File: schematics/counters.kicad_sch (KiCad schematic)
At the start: 28 parts, among them U10 74HC390, U11 74HC390, U12 74HC390, U13 ATF22V10C, U4 74HC08, U5 74HC08, U6 74HC4046, U7 74HC86, U8 74HC390, U9 74HC390

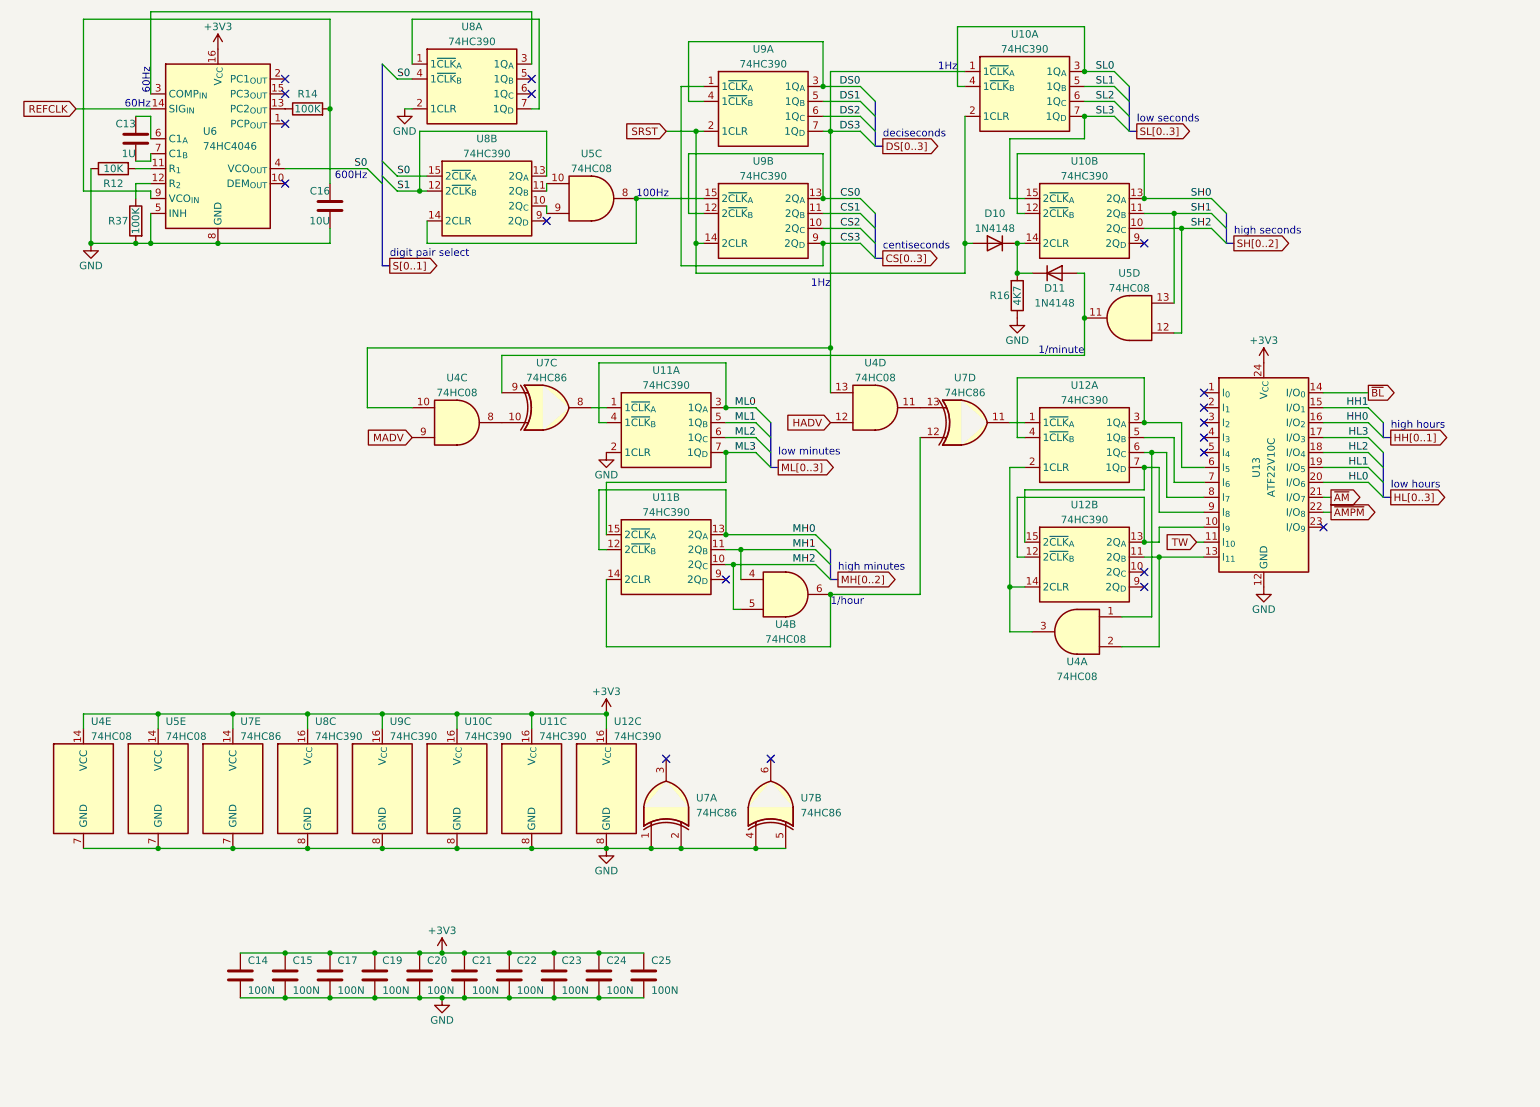
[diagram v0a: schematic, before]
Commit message: started a second version
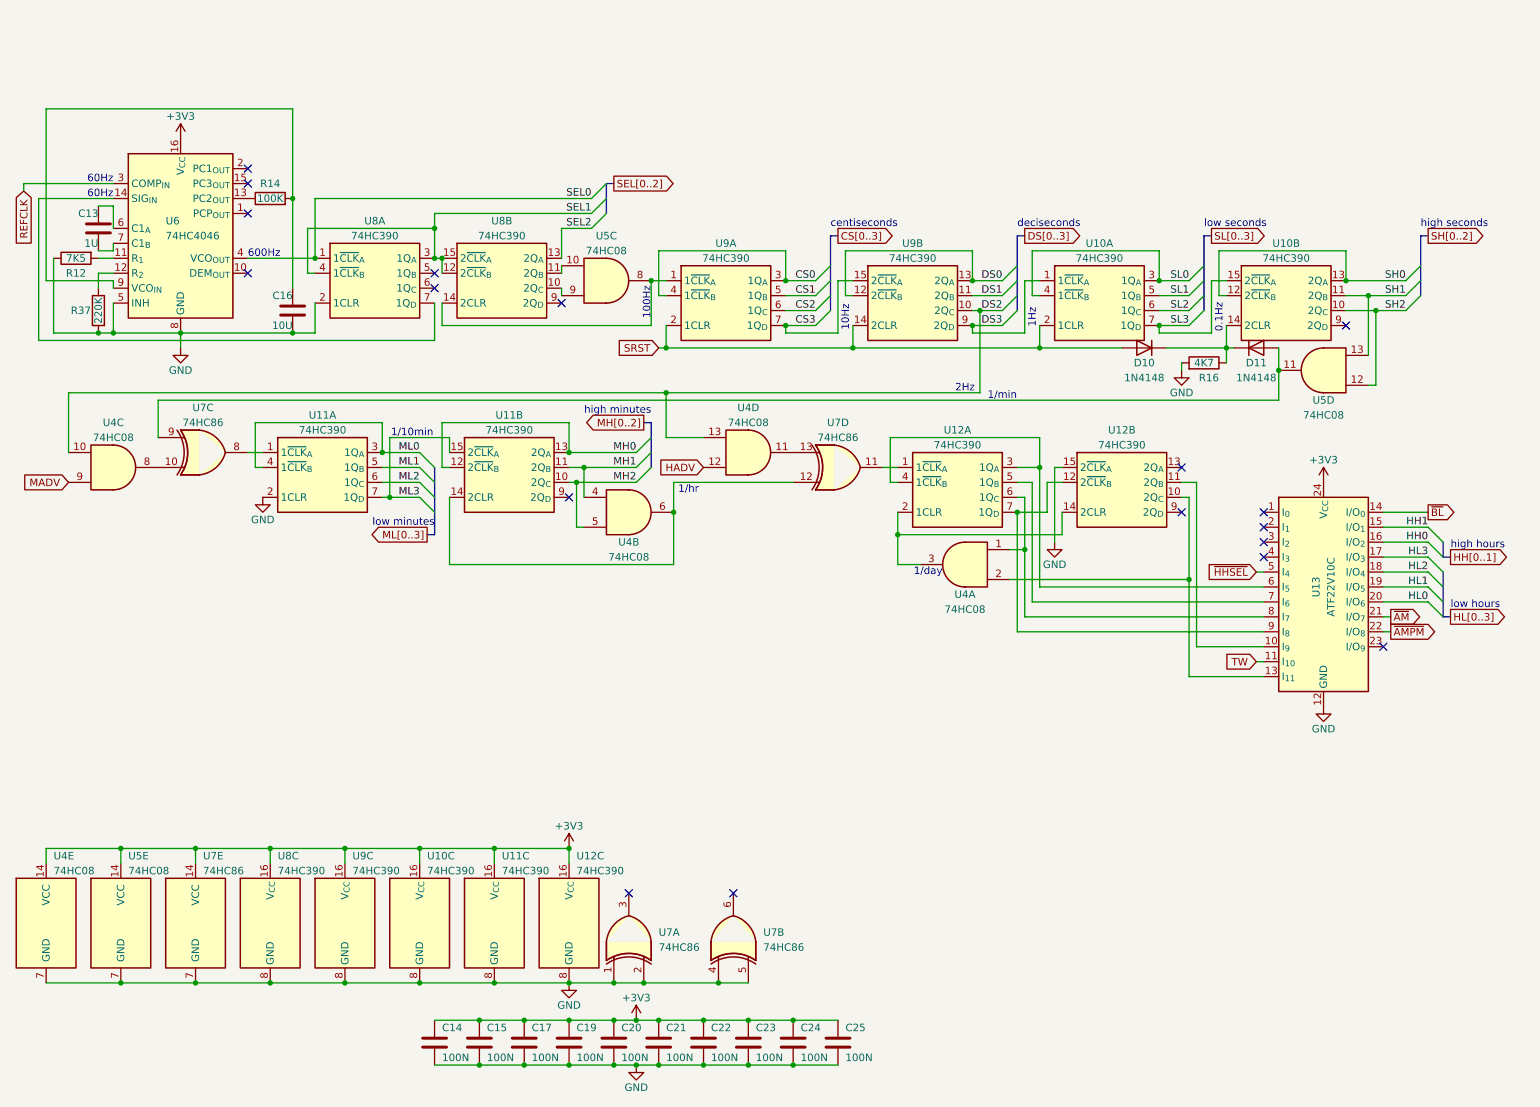
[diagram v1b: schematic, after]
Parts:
- R12: value 10K -> 7K5
- R37: value 100K -> 220K
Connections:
- net CS0: now also U9.3 (1Q_{A}), U9.4 (1~{CLK}_{B}); no longer U9.12 (2~{CLK}_{B}), U9.13 (2Q_{A})
- net CS1: now also U9.5 (1Q_{B}); no longer U9.11 (2Q_{B})
- net CS2: now also U9.6 (1Q_{C}); no longer U9.10 (2Q_{C})
- net CS3: now also U9.15 (2~{CLK}_{A}), U9.7 (1Q_{D}); no longer U9.1 (1~{CLK}_{A}), U9.9 (2Q_{D})
- net DS0: now also U9.12 (2~{CLK}_{B}), U9.13 (2Q_{A}); no longer U9.3 (1Q_{A}), U9.4 (1~{CLK}_{B})
- net DS1: now also U9.11 (2Q_{B}); no longer U9.5 (1Q_{B})
- net DS2: now also U4.10, U4.13, U9.10 (2Q_{C}); no longer U9.6 (1Q_{C})
- net DS3: now also U9.9 (2Q_{D}); no longer U4.10, U4.13, U9.7 (1Q_{D})
- net GND: now also R16.2, U12.15 (2~{CLK}_{A}); no longer R16.1
- net REFCLK: now also U6.3 (COMP_{IN}); no longer U6.14 (SIG_{IN})
- net at U12.10 (2Q_{C}): now also U13.13 (I_{11}), U4.2
- net at U12.7 (1Q_{D}), U13.9 (I_{8}): now also U12.12 (2~{CLK}_{B}); no longer U12.15 (2~{CLK}_{A})
- net at D10.1 (K), D11.1 (K), U10.14 (2CLR): now also R16.1; no longer R16.2
- net at U8.7 (1Q_{D}): now also U6.14 (SIG_{IN}); no longer U8.1 (1~{CLK}_{A})
- net SEL1: now reaches U8.3 (1Q_{A})
- net SEL1: now also U8.12 (2~{CLK}_{B}), U8.15 (2~{CLK}_{A}), U8.4 (1~{CLK}_{B}); no longer U6.3 (COMP_{IN})
- net at U5.8, U8.14 (2CLR): now also U9.1 (1~{CLK}_{A}); no longer U9.15 (2~{CLK}_{A})
- net ~{HHSEL}: now reaches U13.5 (I_{4})
- removed net S0: U6.4 (VCO_{OUT}), U8.15 (2~{CLK}_{A}), U8.4 (1~{CLK}_{B})
- net S1 renamed SEL2
- net SEL2: no longer U8.12 (2~{CLK}_{B})
- new net: U12.11 (2Q_{B}), U13.10 (I_{9})
- new net SEL0: U6.4 (VCO_{OUT}), U8.1 (1~{CLK}_{A})
- now unconnected: U12.13 (2Q_{A})
- no-connect marks 19 -> 18
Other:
- note added: "0.1Hz"
- note added: "1/10min"
- note added: "1/day"
- note added: "1/hr"
- note added: "1/min"
- note added: "10Hz"
- note added: "2Hz"
- note removed: "1/hour"
- note removed: "1/minute"
- note removed: "digit pair select"
- moved on the sheet: C13, C14, C15, C16, C17, C19, C20, C21, C22, C23, C24, C25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
